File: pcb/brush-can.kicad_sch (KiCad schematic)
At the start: 29 parts, among them J1 Conn_01x02_MountingPin, J2 Conn_01x04_MountingPin, J3 Conn_01x04_MountingPin, J8 Conn_01x04_MountingPin, M1 24939, M2 24939, U1 AP62150Z6, U2 NCP176, U4 TJA1044GTK/3, U8 STM32G431KBUx, Y1 24MHz

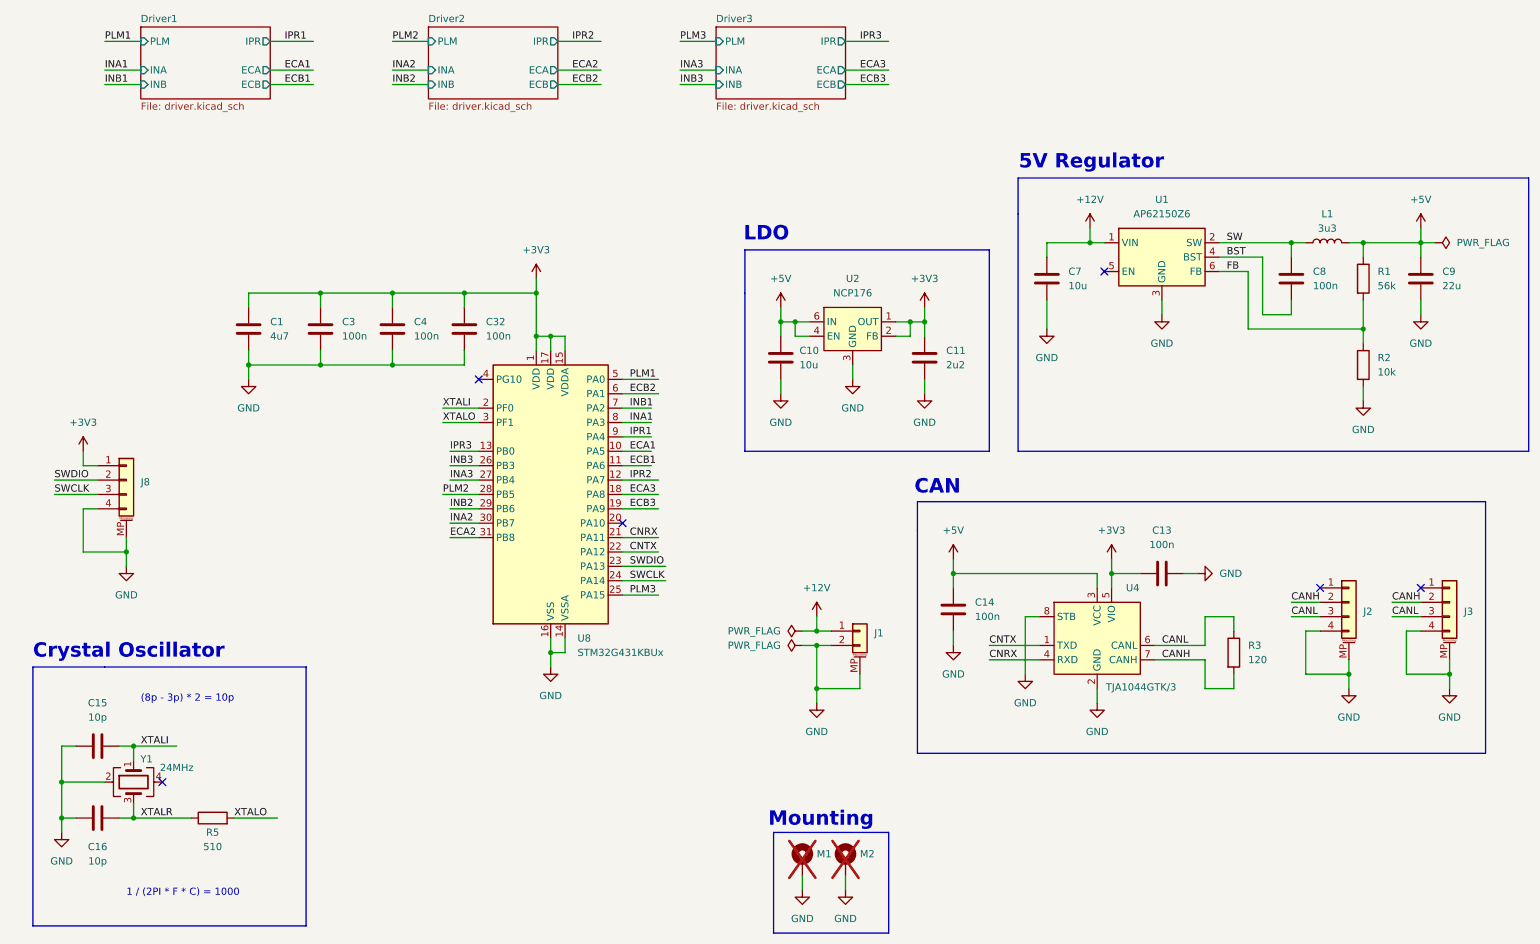
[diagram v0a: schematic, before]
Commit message: Save
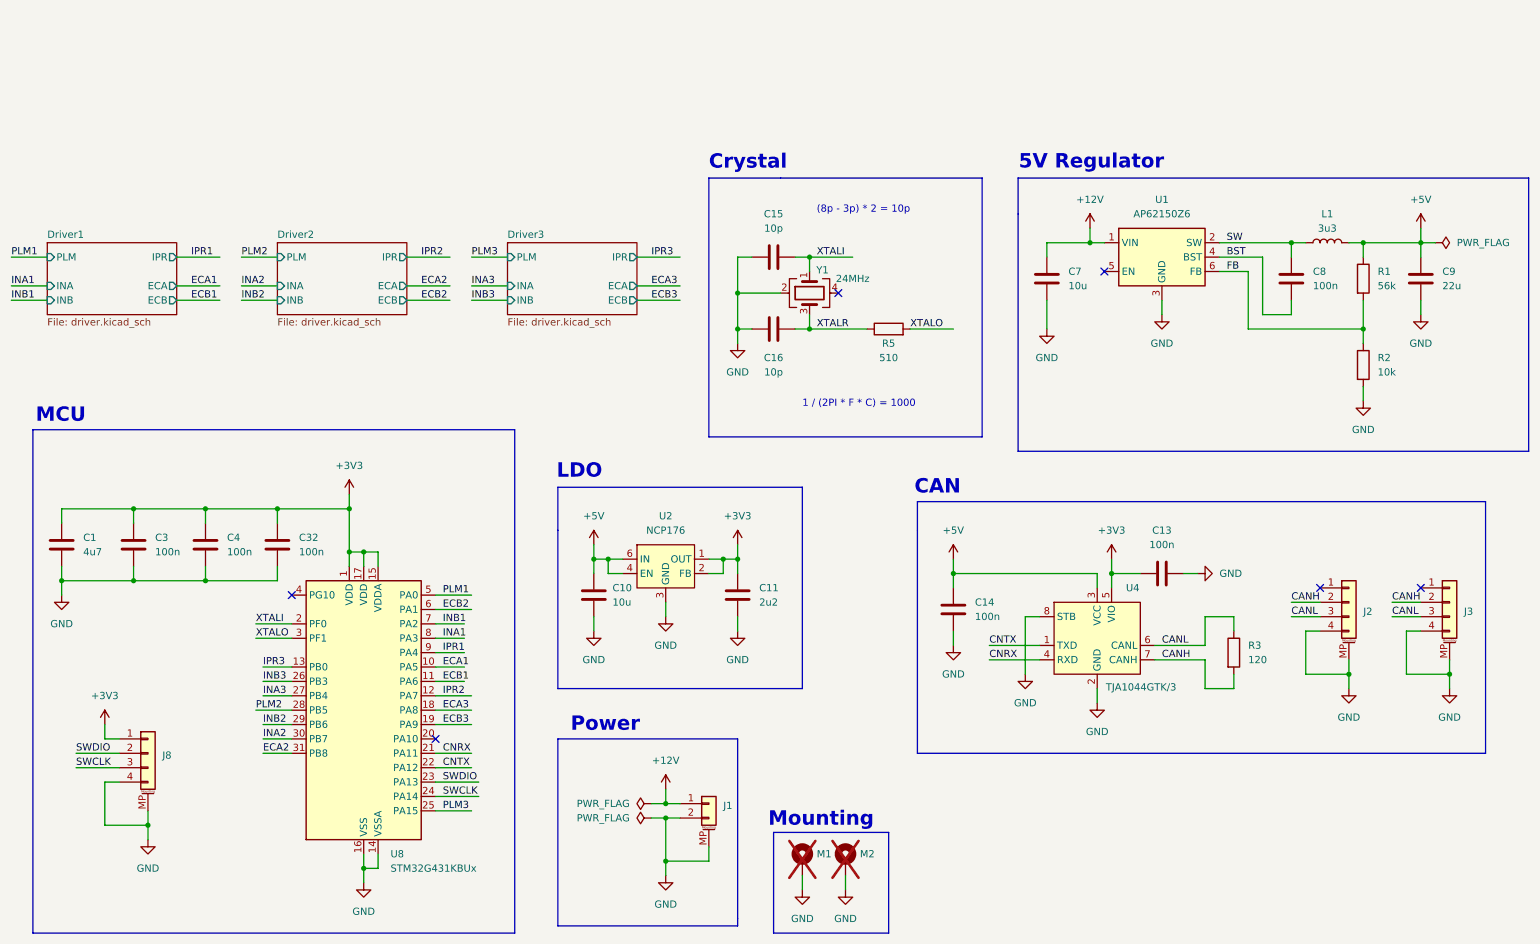
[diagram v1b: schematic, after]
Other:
- note added: "Crystal"
- note added: "MCU"
- note added: "Power"
- note removed: "Crystal Oscillator"
- moved on the sheet: C1, C10, C11, C15, C16, C3, C32, C4, J1, J8, R5, U2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
